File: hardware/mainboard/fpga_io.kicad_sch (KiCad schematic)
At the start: 24 parts, among them U1 LIFCL_40_CABGA400, X1 XO32

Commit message: Add and assign more footprints
Signed-off-by: David Shah <dave@ds0.me>
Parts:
- U1: footprint (none) -> meowality:BGA-400_20x20_17.0x17.0mm
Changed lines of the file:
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@@
       (effects (font (size 1.524 1.524)) (justify left))
     )
-    (property "Footprint" "" (id 2) (at 64.77 43.18 0)
+    (property "Footprint" "meowality:BGA-400_20x20_17.0x17.0mm" (id 2) (at 64.77 43.18 0)
       (effects (font (size 1.524 1.524)) (justify right) hide)
     )
@@
       (effects (font (size 1.524 1.524)) (justify left))
     )
-    (property "Footprint" "" (id 2) (at 179.07 256.54 0)
+    (property "Footprint" "meowality:BGA-400_20x20_17.0x17.0mm" (id 2) (at 179.07 256.54 0)
       (effects (font (size 1.524 1.524)) (justify right) hide)
     )
@@
       (effects (font (size 1.524 1.524)) (justify left))
     )
-    (property "Footprint" "" (id 2) (at 64.77 114.3 0)
+    (property "Footprint" "meowality:BGA-400_20x20_17.0x17.0mm" (id 2) (at 64.77 114.3 0)
       (effects (font (size 1.524 1.524)) (justify right) hide)
     )
@@
       (effects (font (size 1.524 1.524)) (justify left))
     )
-    (property "Footprint" "" (id 2) (at 330.2 156.21 0)
+    (property "Footprint" "meowality:BGA-400_20x20_17.0x17.0mm" (id 2) (at 330.2 156.21 0)
       (effects (font (size 1.524 1.524)) (justify right) hide)
     )
@@
       (effects (font (size 1.524 1.524)) (justify left))
     )
-    (property "Footprint" "" (id 2) (at 68.58 209.55 0)
+    (property "Footprint" "meowality:BGA-400_20x20_17.0x17.0mm" (id 2) (at 68.58 209.55 0)
       (effects (font (size 1.524 1.524)) (justify right) hide)
     )
@@
       (effects (font (size 1.524 1.524)) (justify left))
     )
-    (property "Footprint" "" (id 2) (at 335.28 44.45 0)
+    (property "Footprint" "meowality:BGA-400_20x20_17.0x17.0mm" (id 2) (at 335.28 44.45 0)
       (effects (font (size 1.524 1.524)) (justify right) hide)
     )
@@
       (effects (font (size 1.524 1.524)) (justify left))
     )
-    (property "Footprint" "" (id 2) (at 195.58 149.86 0)
+    (property "Footprint" "meowality:BGA-400_20x20_17.0x17.0mm" (id 2) (at 195.58 149.86 0)
       (effects (font (size 1.524 1.524)) (justify right) hide)
     )
@@
       (effects (font (size 1.524 1.524)) (justify left))
     )
-    (property "Footprint" "" (id 2) (at 176.53 44.45 0)
-      (effects (font (size 1.524 1.524)) (justify right) hide)
-    )
+    (property "Footprint" "meowality:BGA-400_20x20_17.0x17.0mm" (id 2) (at 176.53 44.45 0)
+      (effects (font (size 1.524 1.524)) (justify right) hide)
+    )

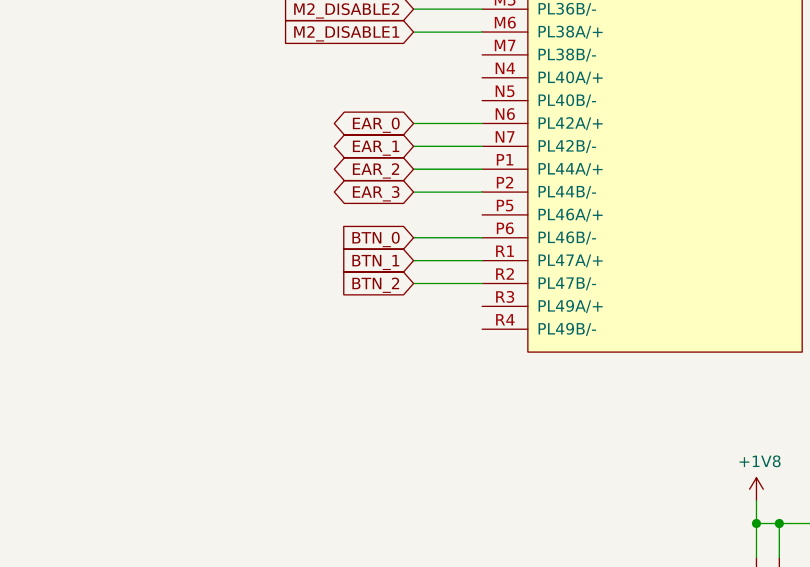
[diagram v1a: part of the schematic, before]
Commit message: Working on layout
Signed-off-by: David Shah <dave@ds0.me>
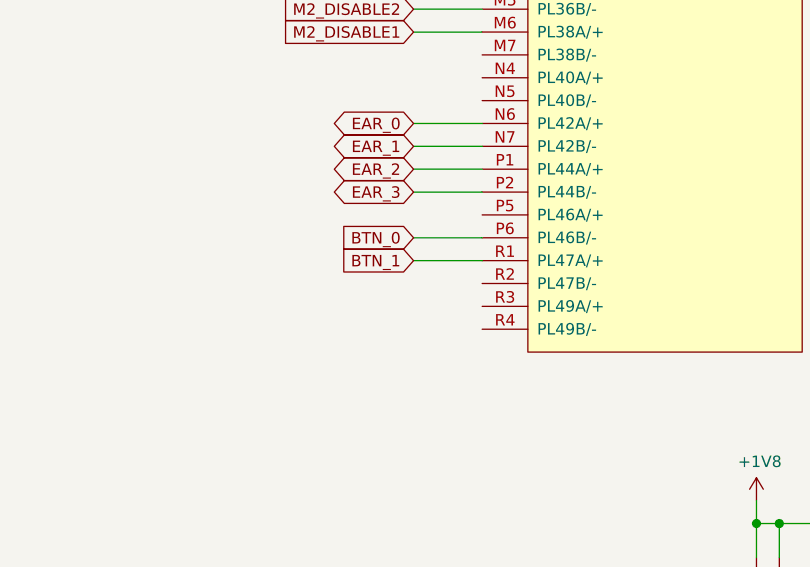
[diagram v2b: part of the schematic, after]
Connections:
- net BTN_2: no longer names the net of U1.R2 (PL47B/-)
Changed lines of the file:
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@@
-    (stroke (width 0) (type solid) (color 0 0 0 0))
-  )
-  (wire (pts (xy 323.85 109.22) (xy 331.47 109.22))
     (stroke (width 0) (type solid) (color 0 0 0 0))
   )
@@
       (effects (font (size 1.27 1.27)) (justify right) hide)
     )
-  )
-  (global_label "BTN_2" (shape input) (at 323.85 109.22 180)
-    (effects (font (size 1.27 1.27)) (justify right))
-    (property "Intersheet References" "${INTERSHEET_REFS}" (id 0) (at 314.1677 109.1406 0)
-      (effects (font (size 1.27 1.27)) (justify right) hide)
-    )
